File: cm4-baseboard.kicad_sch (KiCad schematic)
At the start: 4 parts

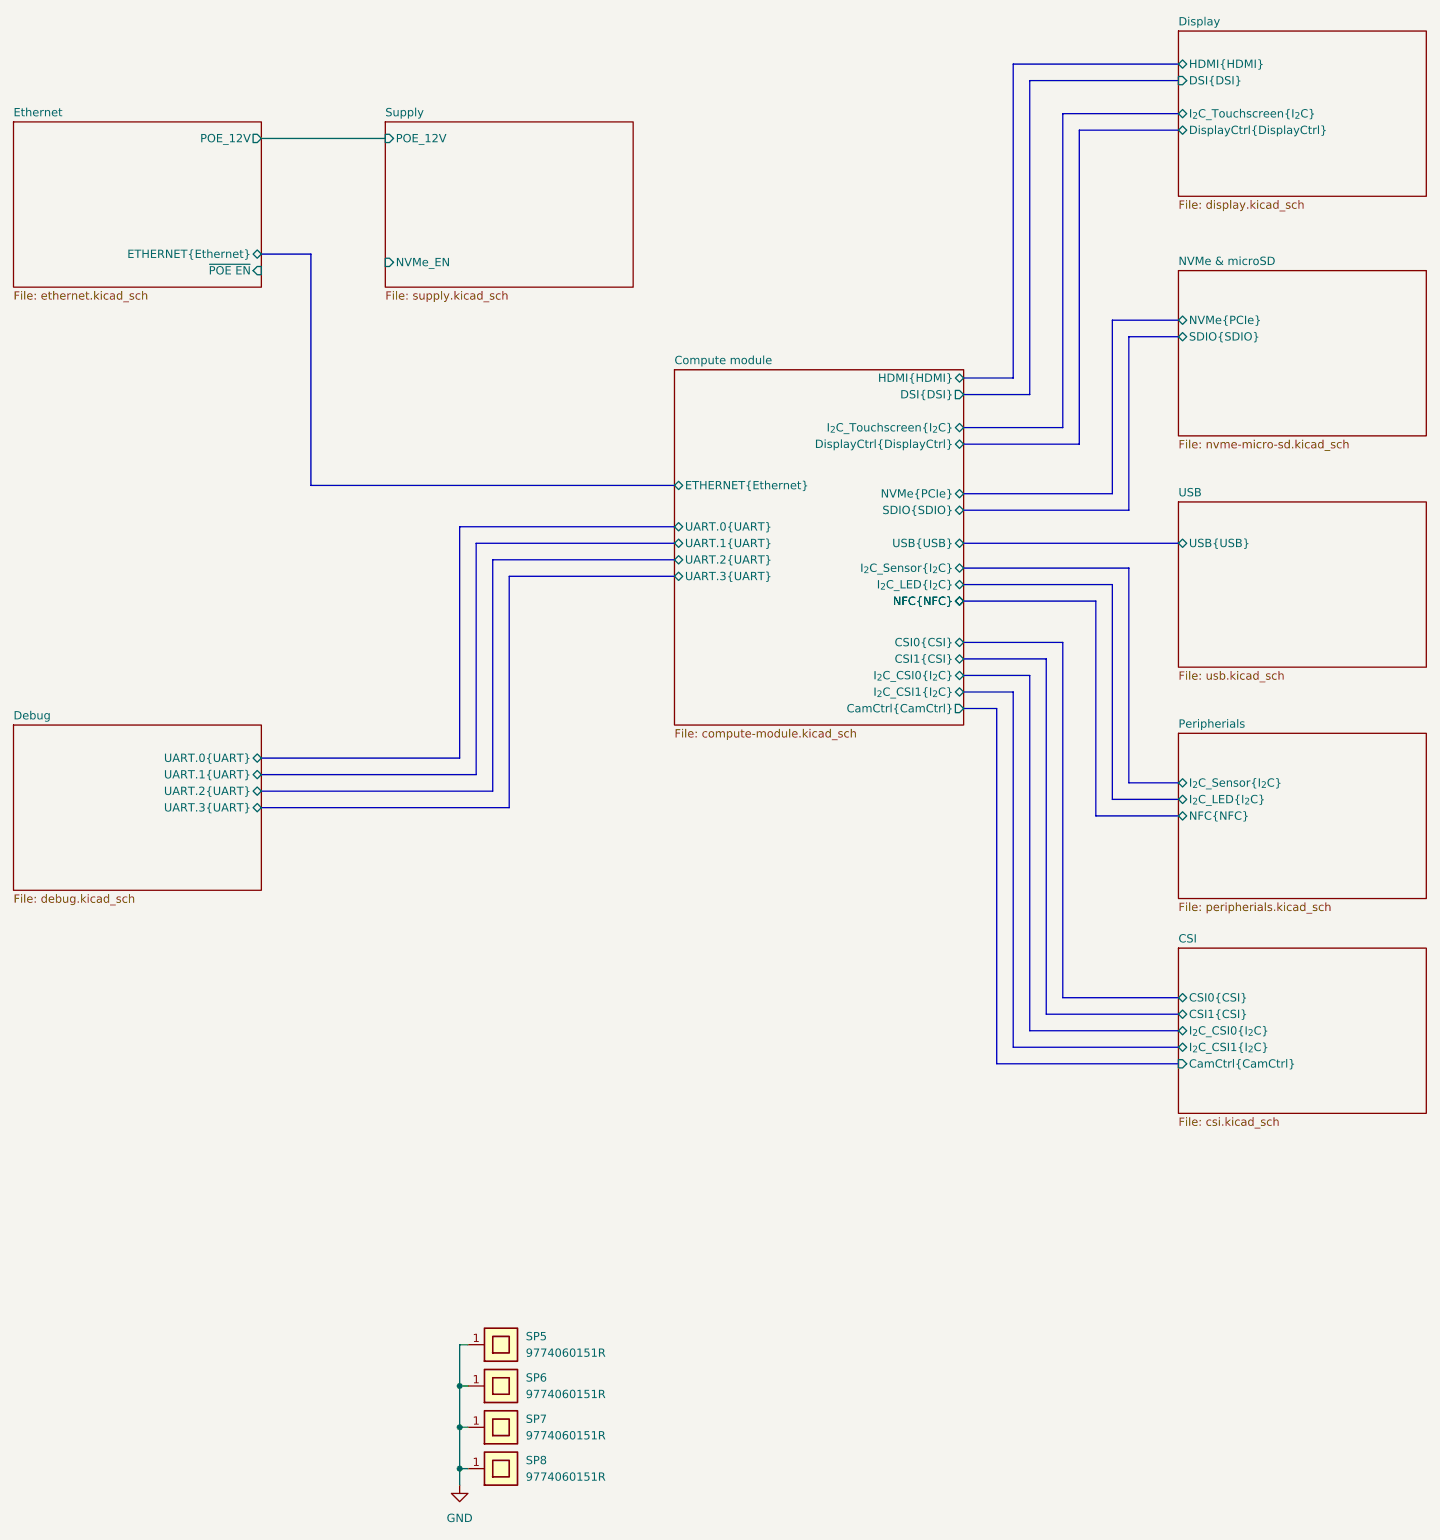
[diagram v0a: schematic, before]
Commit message: [#54447] CM4 connections part 3
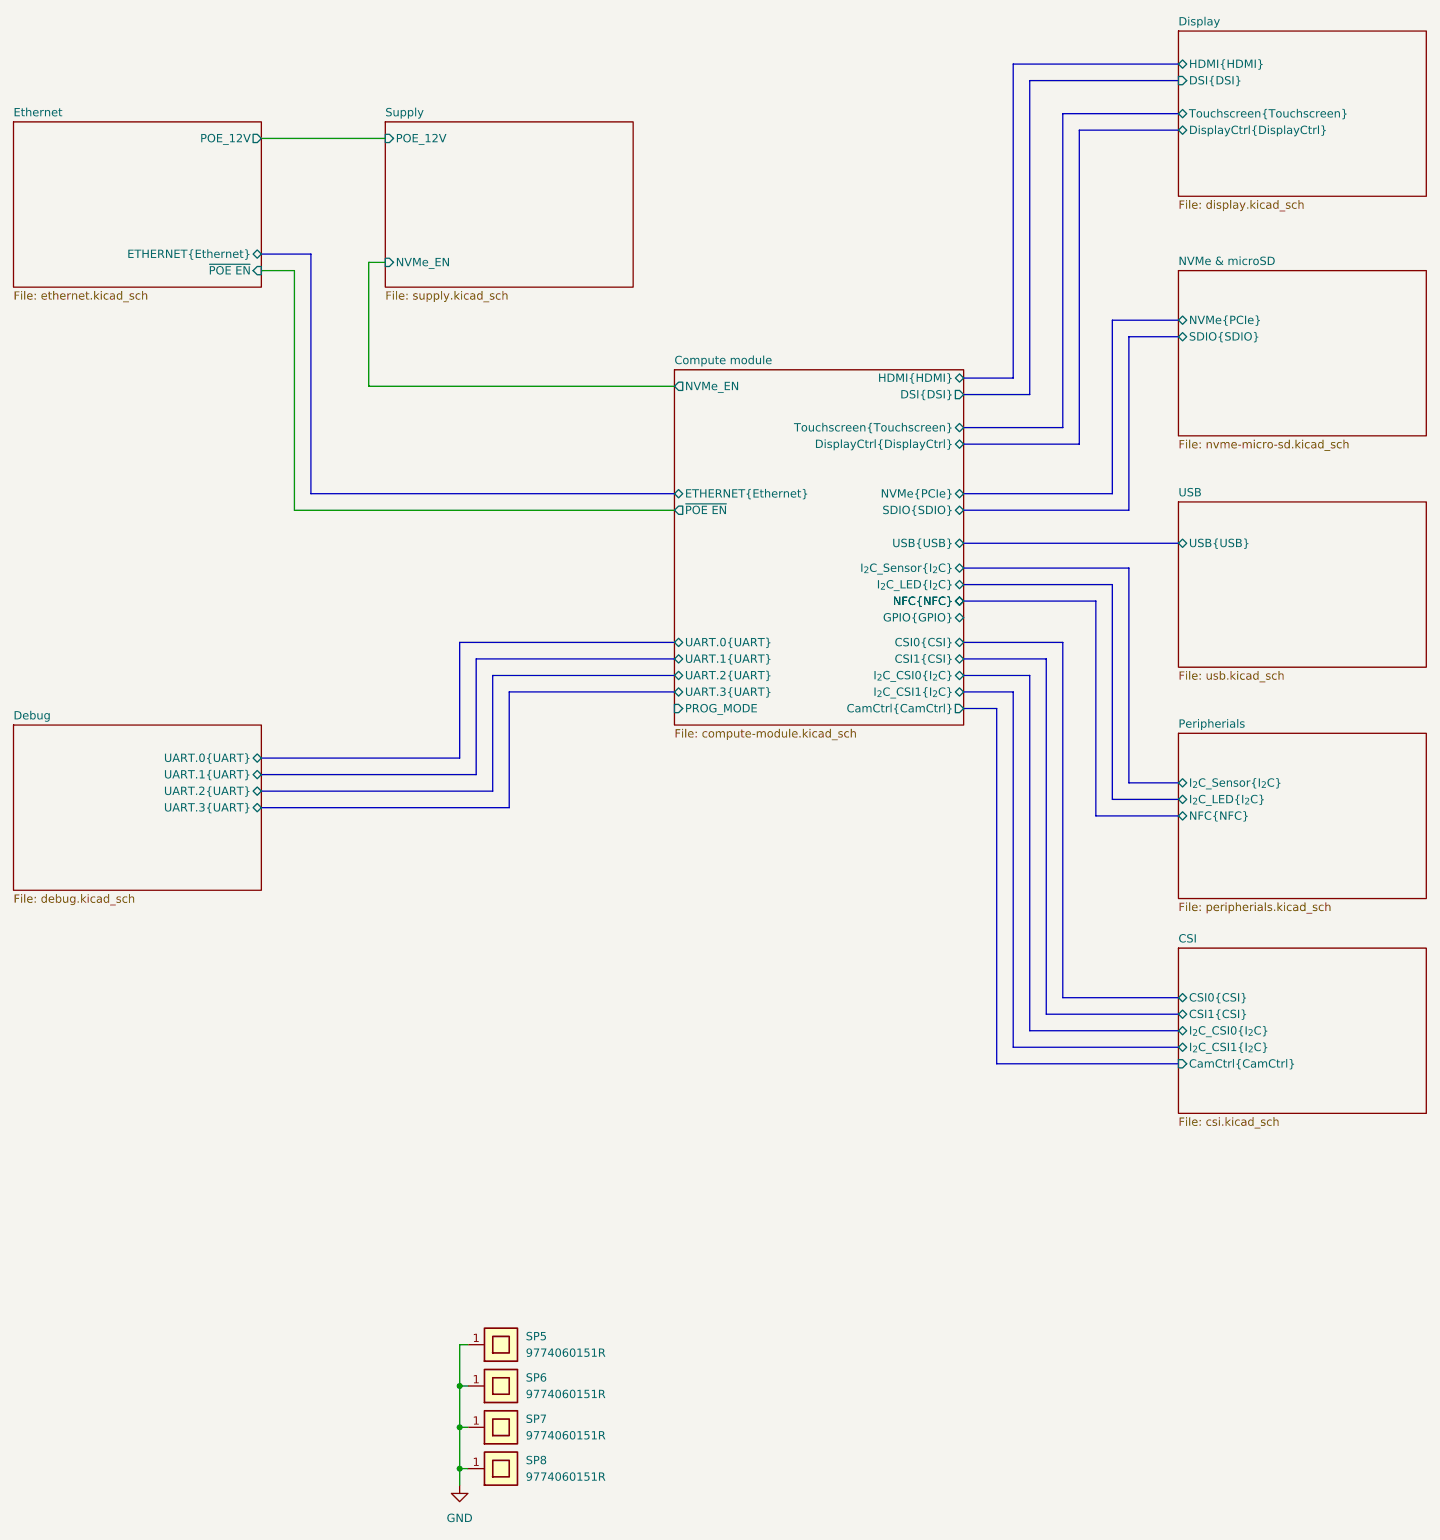
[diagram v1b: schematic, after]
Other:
- sheet Compute module ports: added GPIO{GPIO}, NVMe_EN, PROG_MODE, Touchscreen{Touchscreen}, ~{POE EN}; removed I_{2}C_Touchscreen{I_{2}C}
- sheet Display ports: added Touchscreen{Touchscreen}; removed I_{2}C_Touchscreen{I_{2}C}
